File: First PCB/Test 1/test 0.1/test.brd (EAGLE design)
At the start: 84 x 39.1 mm, 7 parts, among them SW2 B3U-1000P

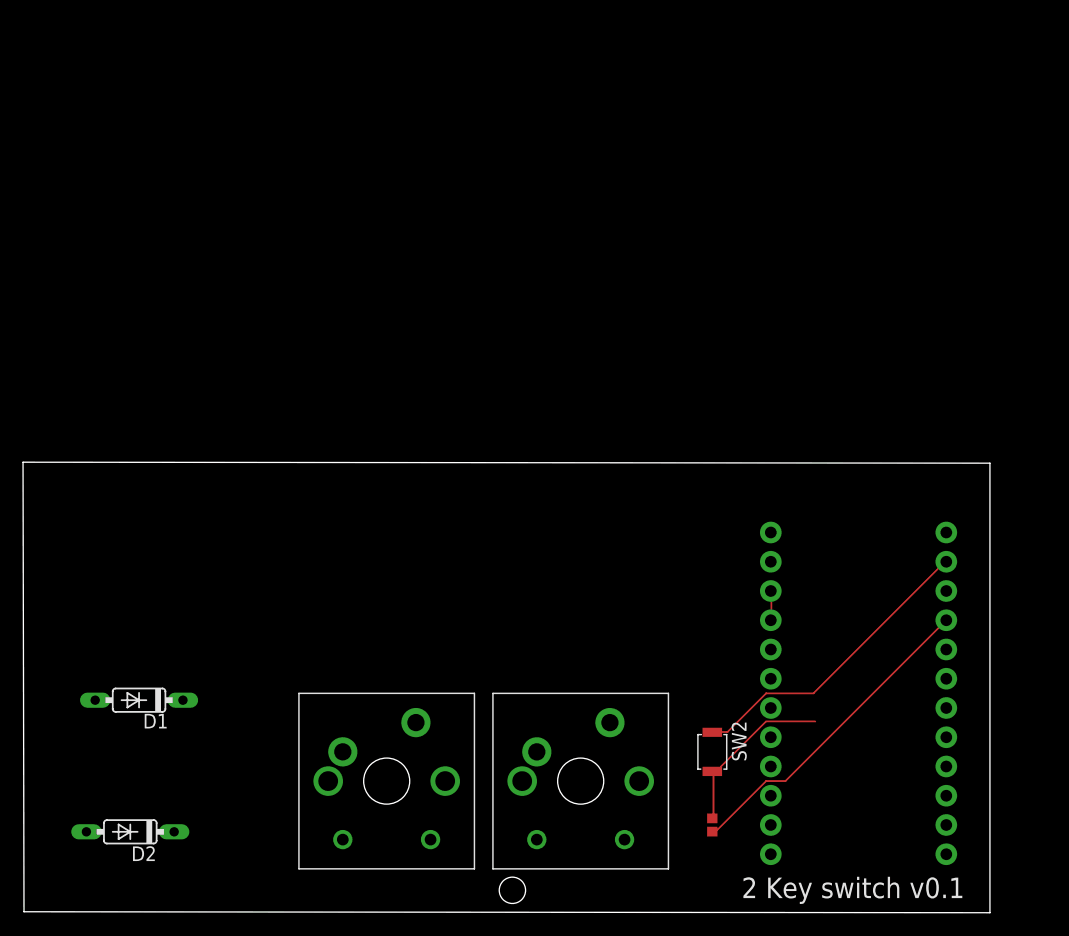
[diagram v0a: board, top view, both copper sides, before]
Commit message: finished board and submitted for review, https://geekhack.org/index.php?topic=102077.0
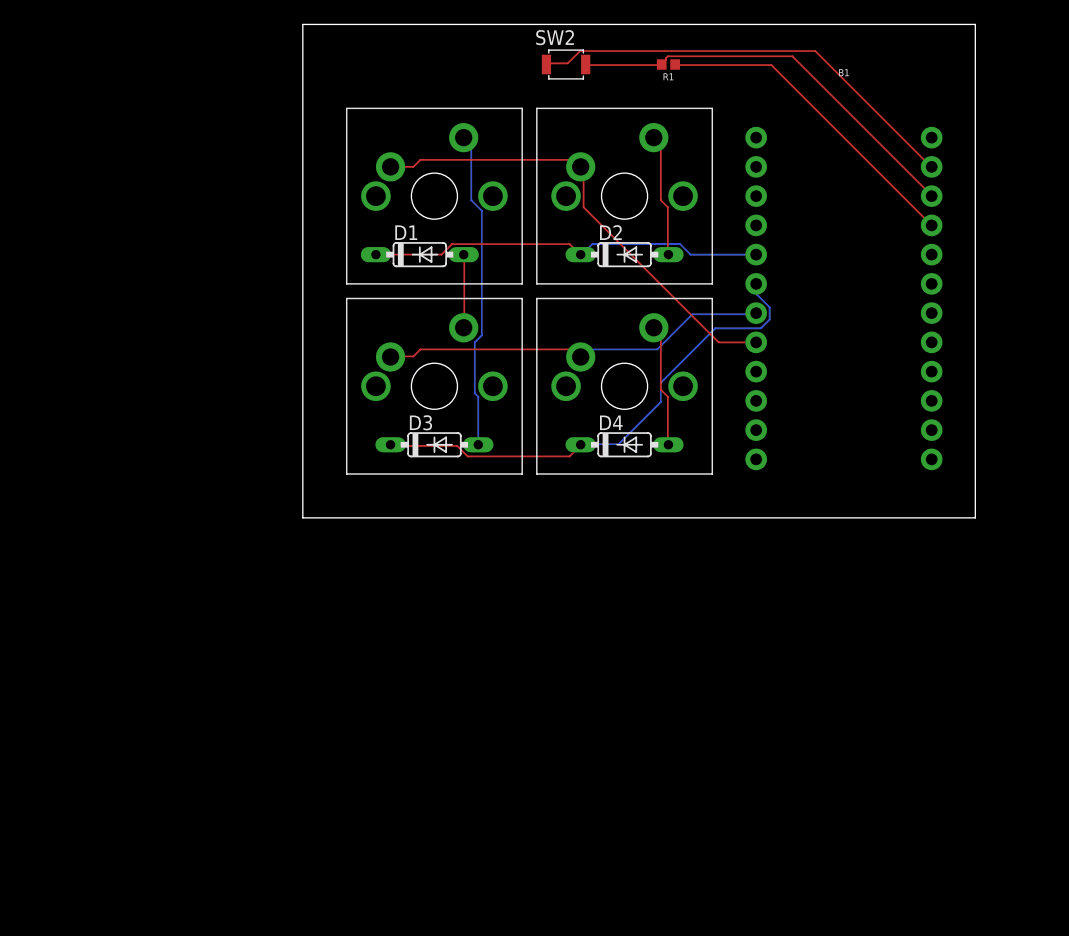
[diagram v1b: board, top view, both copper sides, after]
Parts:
- removed DIODE, DIODE1: CHERRY-MX-DIODE, cherrymx:CHERRY-MX-DIODE
- added D3, D4: 1N4148DO35-7, diode:DO35-7
- added U$1, U$2, U$3, U$4: CHERRY-MX, cherrymx:CHERRY-MX
- moved R1 66.1 mm to (96.5, 96.5), turned to 180 degrees
- moved D2 66.0 mm to (92.7, 80.0), turned to 0 degrees
- moved SW2 61.0 mm to (87.6, 96.5), turned to 0 degrees
- moved D1 45.7 mm to (74.9, 80.0), turned to 0 degrees
- moved B1 34.3 mm to (111.8, 77.5)
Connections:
- new net N$10: D4.A, U$2.SW2
- new net N$12: D3.A, U$3.SW2
- new net N$6: B1.7, U$1.SW1, U$2.SW1
- new net N$8: D2.A, U$4.SW2
- new net N$9: B1.8, U$3.SW1, U$4.SW1
- net N$4: now also B1.5, D1.C, D2.C; no longer B1.6, DIODE.SW1
- net N$5: now also D1.A, U$1.SW2; no longer D2.C, DIODE1.SW1
- net N$7: now also B1.6, D3.C, D4.C; no longer D2.A, DIODE.D1
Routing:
- net N$7: track 0.00 -> 42.9 mm
- net N$9: track 0.00 -> 40.5 mm
- net N$4: track 0.11 -> 34.5 mm
- net N$6: track 0.00 -> 33.9 mm
- net N$12: track 0.00 -> 27.7 mm
- net N$1: track 15.0 -> 35.5 mm
- net N$3: track 26.4 -> 38.1 mm
- net N$8: track 0.00 -> 10.7 mm
- net N$10: track 0.00 -> 10.7 mm
- net N$5: track 0.00 -> 6.41 mm
- net GND: track 2.58 -> 0.00 mm
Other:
- board size 84 x 39.1 mm -> 58.4 x 42.9 mm
- board text removed: ""lets see if this works""
- board text removed: "-MintCollie"
- board text removed: "2 Key switch v0.1"
- board text removed: "C:/Users/Mint/Pictures/test2.bmp"
